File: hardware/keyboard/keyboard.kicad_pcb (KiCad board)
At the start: 2 copper layers, 38 parts, among them J1 Conn_01x08_Pin, J2 Conn_01x08_Pin, J3 Conn_01x08_Pin, J4 Conn_01x08_Pin, J5 Conn_01x26_Socket, J6 Conn_01x12_Pin, Q1 PC817C, Q10 PC817C, Q11 PC817C, Q12 PC817C, Q13 PC817C, Q14 PC817C, Q15 PC817C, Q16 PC817C, Q17 PC817C, Q18 PC817C, Q19 PC817C, Q2 PC817C, Q20 PC817C, Q21 PC817C, Q22 PC817C, Q23 PC817C, Q24 PC817C, Q25 PC817C, Q26 PC817C, Q27 PC817C, Q28 PC817C, Q29 PC817C, Q3 PC817C, Q30 PC817C, Q31 PC817C, Q32 PC817C, Q4 PC817C, Q5 PC817C, Q6 PC817C, Q7 PC817C, Q8 PC817C, Q9 PC817C

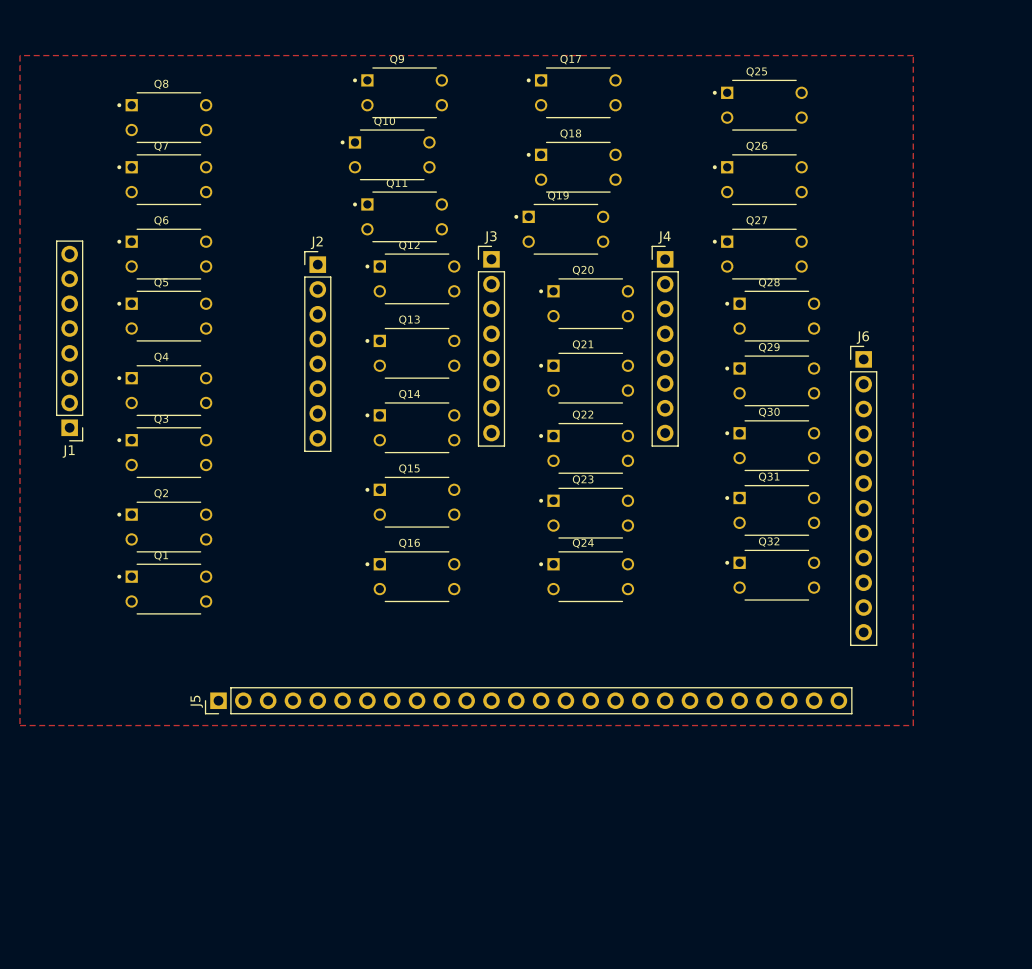
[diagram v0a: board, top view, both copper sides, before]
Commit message: Update
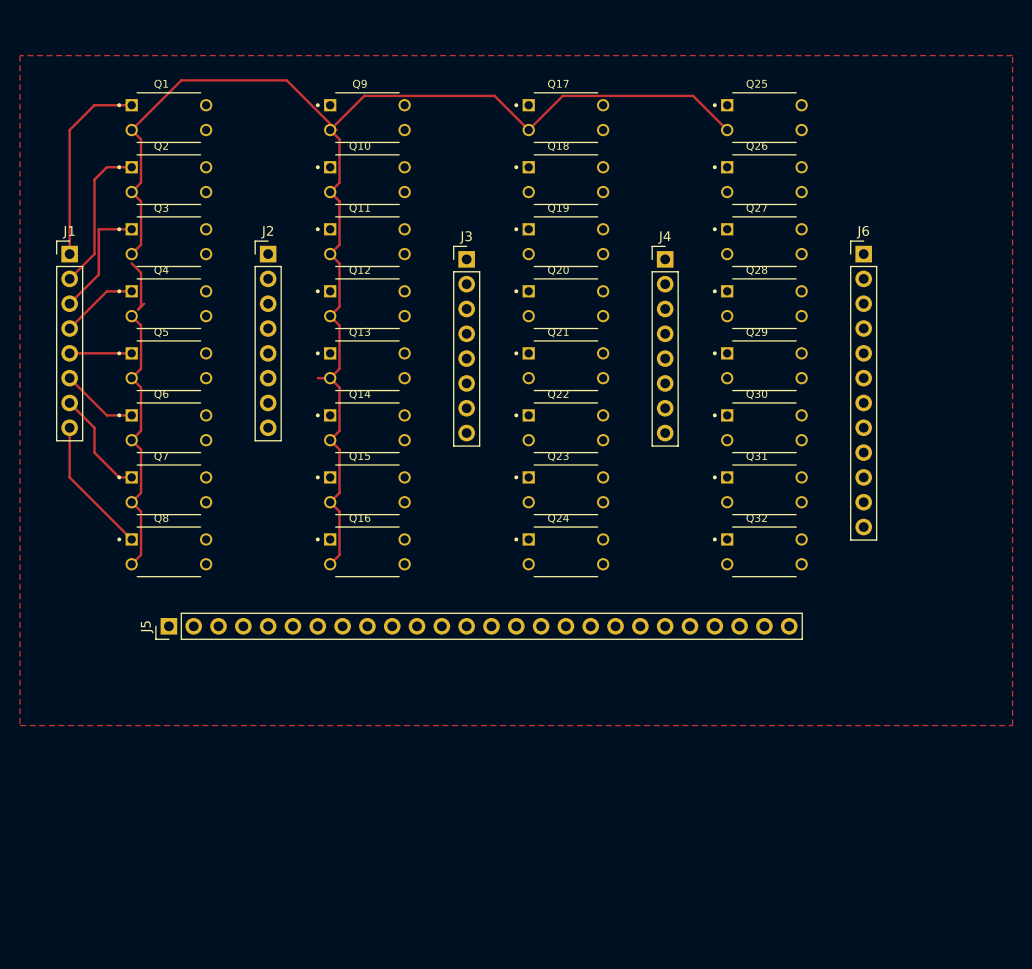
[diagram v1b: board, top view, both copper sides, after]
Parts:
- moved Q1 48.3 mm to (99.1, 47.0)
- moved Q8 44.4 mm to (99.1, 91.4)
- moved Q2 35.6 mm to (99.1, 53.3)
- moved Q7 31.8 mm to (99.1, 85.1)
- moved Q3 21.6 mm to (99.1, 59.7)
- moved J1 17.8 mm to (88.9, 61.0), turned to 0 degrees
- moved Q6 17.8 mm to (99.1, 78.7)
- moved J6 10.8 mm to (170.2, 61.0)
- moved J5 9.16 mm to (99.1, 99.1)
- moved Q4 8.89 mm to (99.1, 66.0)
- moved Q12 5.68 mm to (119.4, 66.0)
- moved Q16 5.68 mm to (119.4, 91.4)
- moved Q13 5.24 mm to (119.4, 72.4)
- moved Q15 5.24 mm to (119.4, 85.1)
- moved J2 5.19 mm to (109.2, 61.0)
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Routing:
- net Net-(Q1-Pad2): track 0.00 -> 166.3 mm
- net Net-(J1-Pin_1): track 0.00 -> 20.1 mm
- net Net-(J1-Pin_2): track 0.00 -> 15.5 mm
- net Net-(J1-Pin_8): track 0.00 -> 14.1 mm
- net Net-(J1-Pin_3): track 0.00 -> 12.2 mm
- net Net-(J1-Pin_7): track 0.00 -> 11.0 mm
- net Net-(J1-Pin_6): track 0.00 -> 7.93 mm
- net Net-(J1-Pin_4): track 0.00 -> 7.93 mm
- net Net-(J1-Pin_5): track 0.00 -> 6.35 mm
- net (no net): track 0.00 -> 6.07 mm

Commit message: Updates v1.0
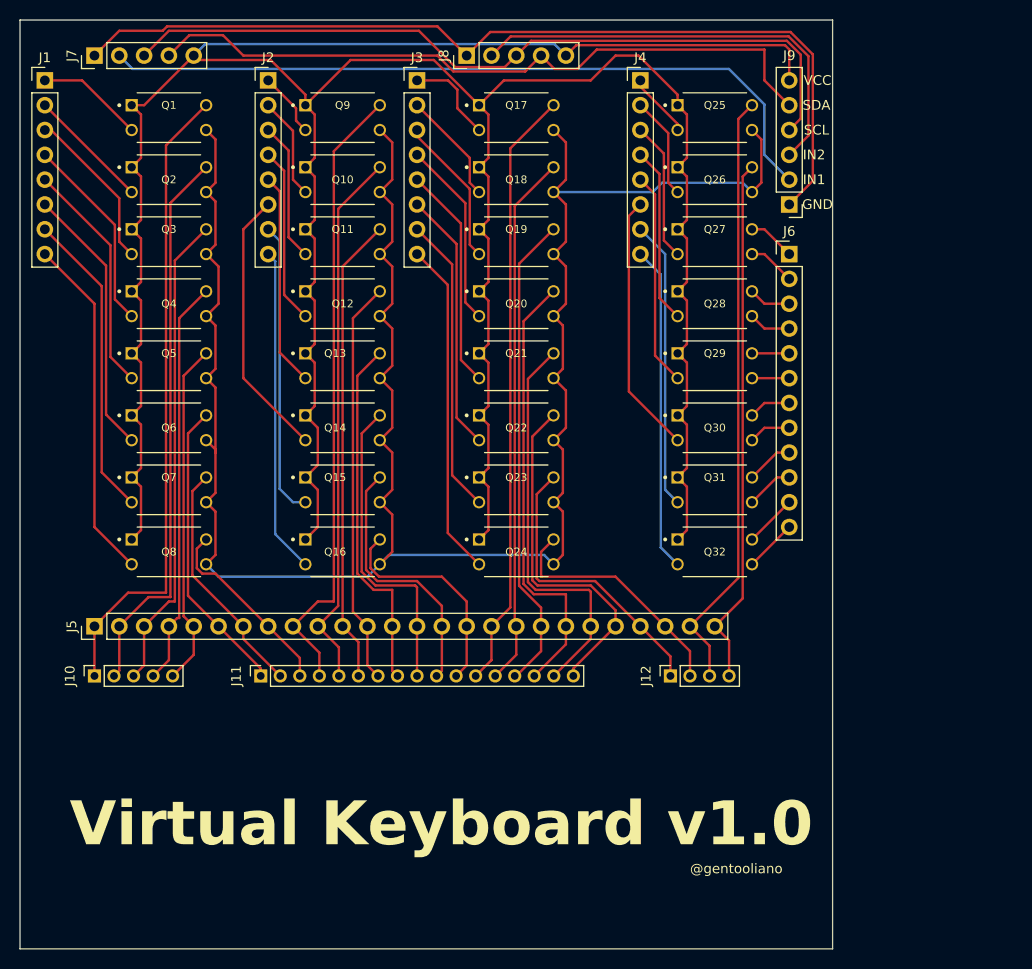
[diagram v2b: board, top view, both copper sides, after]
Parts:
- added J10: Conn_01x05_Socket, Connector_PinSocket_2.00mm:PinSocket_1x05_P2.00mm_Vertical, F.Cu at (91.4, 104.1)
- added J11: Conn_01x17_Socket, Connector_PinSocket_2.00mm:PinSocket_1x17_P2.00mm_Vertical, F.Cu at (108.5, 104.1)
- added J12: Conn_01x04_Socket, Connector_PinSocket_2.00mm:PinSocket_1x04_P2.00mm_Vertical, F.Cu at (150.4, 104.1)
- added J7: Conn_01x05_Pin, Connector_PinHeader_2.54mm:PinHeader_1x05_P2.54mm_Vertical, F.Cu at (91.4, 40.6)
- added J8: Conn_01x05_Pin, Connector_PinHeader_2.54mm:PinHeader_1x05_P2.54mm_Vertical, F.Cu at (129.5, 40.6)
- added J9: Conn_01x06_Pin, Connector_PinHeader_2.54mm:PinHeader_1x06_P2.54mm_Vertical, F.Cu at (162.6, 55.9)
- moved J3 19.0 mm to (124.5, 43.2)
- moved J4 18.5 mm to (147.3, 43.2)
- moved J1 18.0 mm to (86.4, 43.2)
- moved J2 17.8 mm to (109.2, 43.2)
- moved J5 7.62 mm to (91.4, 99.1)
- moved J6 7.62 mm to (162.6, 61.0)
- moved Q25 5.08 mm to (154.9, 47.0)
- moved Q26 5.08 mm to (154.9, 53.3)
- moved Q27 5.08 mm to (154.9, 59.7)
- moved Q28 5.08 mm to (154.9, 66.0)
- moved Q29 5.08 mm to (154.9, 72.4)
- moved Q30 5.08 mm to (154.9, 78.7)
- moved Q31 5.08 mm to (154.9, 85.1)
- moved Q32 5.08 mm to (154.9, 91.4)
- moved Q17 5.08 mm to (134.6, 47.0)
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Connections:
- Q1 pad 1: Net-(J1-Pin_1) -> Net-(J7-Pin_5)
- Q1 pad 2: Net-(Q1-Pad2) -> Net-(J1-Pin_1)
- Q10 pad 1: Net-(J2-Pin_2) -> Net-(J7-Pin_5)
- Q10 pad 2: Net-(Q1-Pad2) -> Net-(J2-Pin_2)
- Q11 pad 1: Net-(J2-Pin_3) -> Net-(J7-Pin_5)
- Q11 pad 2: Net-(Q1-Pad2) -> Net-(J2-Pin_3)
- Q12 pad 1: Net-(J2-Pin_4) -> Net-(J7-Pin_5)
- Q12 pad 2: Net-(Q1-Pad2) -> Net-(J2-Pin_4)
- Q13 pad 1: Net-(J2-Pin_5) -> Net-(J7-Pin_5)
- Q13 pad 2: Net-(Q1-Pad2) -> Net-(J2-Pin_5)
- Q14 pad 1: Net-(J2-Pin_6) -> Net-(J7-Pin_5)
- Q14 pad 2: Net-(Q1-Pad2) -> Net-(J2-Pin_6)
- Q15 pad 1: Net-(J2-Pin_7) -> Net-(J7-Pin_5)
- Q15 pad 2: Net-(Q1-Pad2) -> Net-(J2-Pin_7)
- Q16 pad 1: Net-(J2-Pin_8) -> Net-(J7-Pin_5)
- Q16 pad 2: Net-(Q1-Pad2) -> Net-(J2-Pin_8)
- Q17 pad 1: Net-(J3-Pin_1) -> Net-(J7-Pin_5)
- Q17 pad 2: Net-(Q1-Pad2) -> Net-(J3-Pin_1)
- Q18 pad 1: Net-(J3-Pin_2) -> Net-(J7-Pin_5)
- Q18 pad 2: Net-(Q1-Pad2) -> Net-(J3-Pin_2)
- Q19 pad 1: Net-(J3-Pin_3) -> Net-(J7-Pin_5)
- Q19 pad 2: Net-(Q1-Pad2) -> Net-(J3-Pin_3)
- Q2 pad 1: Net-(J1-Pin_2) -> Net-(J7-Pin_5)
- Q2 pad 2: Net-(Q1-Pad2) -> Net-(J1-Pin_2)
- Q20 pad 1: Net-(J3-Pin_4) -> Net-(J7-Pin_5)
- Q20 pad 2: Net-(Q1-Pad2) -> Net-(J3-Pin_4)
- Q21 pad 1: Net-(J3-Pin_5) -> Net-(J7-Pin_5)
- Q21 pad 2: Net-(Q1-Pad2) -> Net-(J3-Pin_5)
- Q22 pad 1: Net-(J3-Pin_6) -> Net-(J7-Pin_5)
- Q22 pad 2: Net-(Q1-Pad2) -> Net-(J3-Pin_6)
- Q23 pad 1: Net-(J3-Pin_7) -> Net-(J7-Pin_5)
- Q23 pad 2: Net-(Q1-Pad2) -> Net-(J3-Pin_7)
- Q24 pad 1: Net-(J3-Pin_8) -> Net-(J7-Pin_5)
- Q24 pad 2: Net-(Q1-Pad2) -> Net-(J3-Pin_8)
- Q25 pad 1: Net-(J4-Pin_1) -> Net-(J7-Pin_5)
- Q25 pad 2: Net-(Q1-Pad2) -> Net-(J4-Pin_1)
- Q26 pad 1: Net-(J4-Pin_2) -> Net-(J7-Pin_5)
- Q26 pad 2: Net-(Q1-Pad2) -> Net-(J4-Pin_2)
- Q27 pad 1: Net-(J4-Pin_3) -> Net-(J7-Pin_5)
- Q27 pad 2: Net-(Q1-Pad2) -> Net-(J4-Pin_3)
- Q28 pad 1: Net-(J4-Pin_4) -> Net-(J7-Pin_5)
- Q28 pad 2: Net-(Q1-Pad2) -> Net-(J4-Pin_4)
- Q29 pad 1: Net-(J4-Pin_5) -> Net-(J7-Pin_5)
- Q29 pad 2: Net-(Q1-Pad2) -> Net-(J4-Pin_5)
- Q3 pad 1: Net-(J1-Pin_3) -> Net-(J7-Pin_5)
- Q3 pad 2: Net-(Q1-Pad2) -> Net-(J1-Pin_3)
- Q30 pad 1: Net-(J4-Pin_6) -> Net-(J7-Pin_5)
- Q30 pad 2: Net-(Q1-Pad2) -> Net-(J4-Pin_6)
- Q31 pad 1: Net-(J4-Pin_7) -> Net-(J7-Pin_5)
- Q31 pad 2: Net-(Q1-Pad2) -> Net-(J4-Pin_7)
- Q32 pad 1: Net-(J4-Pin_8) -> Net-(J7-Pin_5)
- Q32 pad 2: Net-(Q1-Pad2) -> Net-(J4-Pin_8)
- Q4 pad 1: Net-(J1-Pin_4) -> Net-(J7-Pin_5)
- Q4 pad 2: Net-(Q1-Pad2) -> Net-(J1-Pin_4)
- Q5 pad 1: Net-(J1-Pin_5) -> Net-(J7-Pin_5)
- Q5 pad 2: Net-(Q1-Pad2) -> Net-(J1-Pin_5)
- Q6 pad 1: Net-(J1-Pin_6) -> Net-(J7-Pin_5)
- Q6 pad 2: Net-(Q1-Pad2) -> Net-(J1-Pin_6)
- Q7 pad 1: Net-(J1-Pin_7) -> Net-(J7-Pin_5)
- Q7 pad 2: Net-(Q1-Pad2) -> Net-(J1-Pin_7)
- Q8 pad 1: Net-(J1-Pin_8) -> Net-(J7-Pin_5)
- Q8 pad 2: Net-(Q1-Pad2) -> Net-(J1-Pin_8)
- Q9 pad 1: Net-(J2-Pin_1) -> Net-(J7-Pin_5)
- Q9 pad 2: Net-(Q1-Pad2) -> Net-(J2-Pin_1)
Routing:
- net Net-(J7-Pin_5): track 0.00 -> 335.6 mm
- net Net-(Q1-Pad3): track 0.00 -> 219.6 mm
- net Net-(Q1-Pad2): track 166.3 -> 0.00 mm
- net Net-(J7-Pin_1): track 0.00 -> 94.3 mm
- net Net-(J7-Pin_3): track 0.00 -> 79.7 mm
- net Net-(J7-Pin_2): track 0.00 -> 76.9 mm
- net Net-(J7-Pin_4): track 0.00 -> 72.2 mm
- net Net-(J10-Pin_1): track 0.00 -> 65.4 mm
- net Net-(J11-Pin_4): track 0.00 -> 64.2 mm
- net Net-(J12-Pin_3): track 0.00 -> 61.9 mm
- net Net-(J11-Pin_12): track 0.00 -> 61.7 mm
- net Net-(J10-Pin_2): track 0.00 -> 57.3 mm
- net Net-(J11-Pin_5): track 0.00 -> 55.6 mm
- net Net-(J11-Pin_13): track 0.00 -> 54.4 mm
- net Net-(J12-Pin_4): track 0.00 -> 54.3 mm
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- removed copper zone on F.Cu, net (none)
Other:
- board outline added: 83.2 x 95.1 mm
- board text added: "@gentooliano"
- board text added: "GND"
- board text added: "IN1"
- board text added: "IN2"
- board text added: "SCL"
- board text added: "SDA"
- board text added: "VCC"
- board text added: "Virtual Keyboard v1.0"
